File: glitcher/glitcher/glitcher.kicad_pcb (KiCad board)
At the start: 4 copper layers, 165.1 x 96.5 mm, 81 parts, among them J1 Barrel_Jack, J2 Conn_01x06, J3 Conn_01x03, J4 Conn_01x03, J5 Conn_01x03, J6 Conn_01x03, J7 Conn_01x03, SW1_1V8_OUT1 SW_DPDT_x2, SW2_1V2_OUT1 SW_DPDT_x2, SW3_VADJ_OUT1 SW_DPDT_x2, SW4_3V3_OUT1 SW_DPDT_x2, SW5_2V5_OUT1 SW_DPDT_x2, U1 SC0915, U2 CMOD_A7, U3 max4619cpe+, U4_1V8_OUT1 LD1117S18TR_SOT223, U5_1V2_OUT1 LD1117S12TR_SOT223, U6_VADJ_OUT1 NCP1117-ADJ_SOT223, U7_3V3_OUT1 LD1117S33TR_SOT223, U8_2V5_OUT1 LD1117S25TR_SOT223, U9_3V3ALWAYS1 LD1117S33TR_SOT223

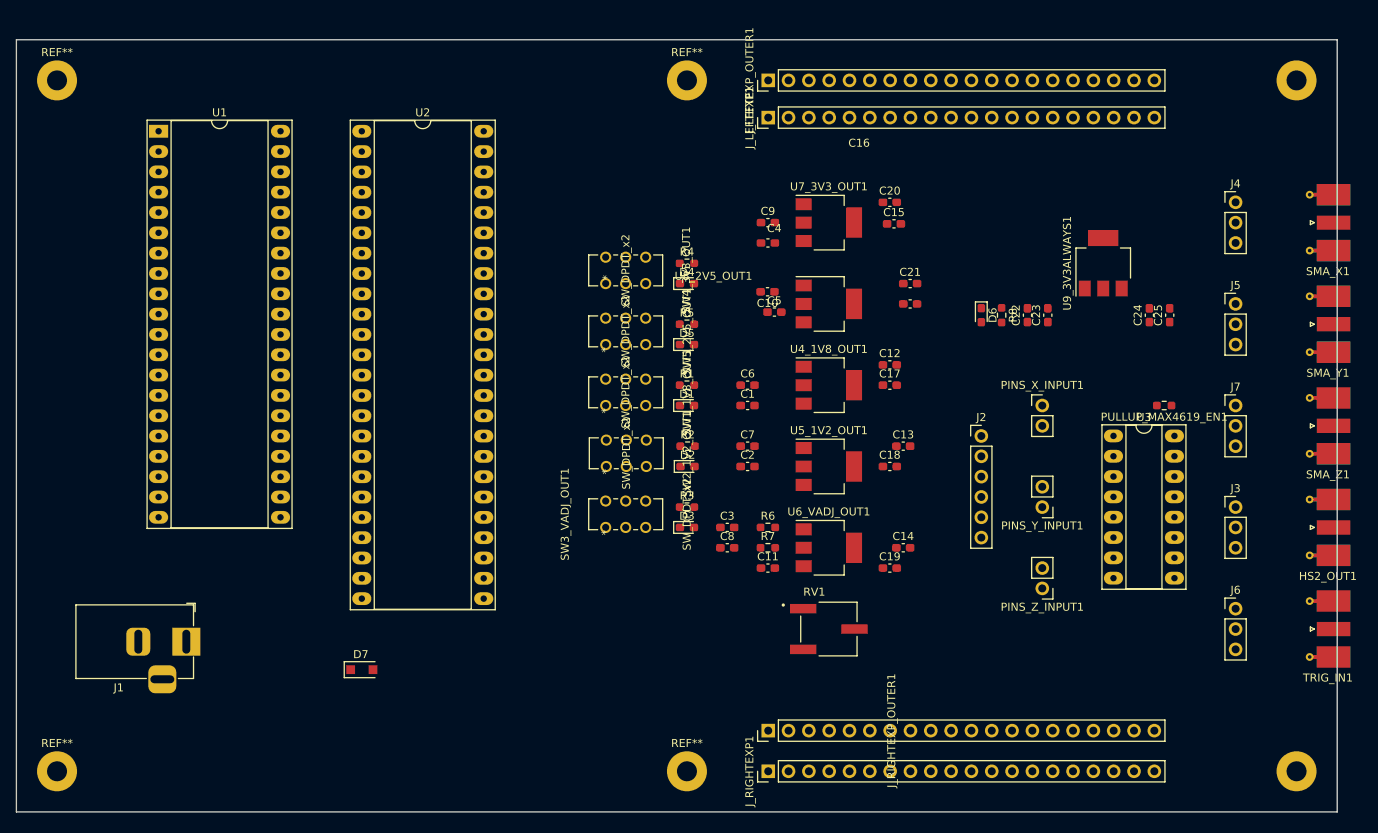
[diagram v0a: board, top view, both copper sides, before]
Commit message: lolsave
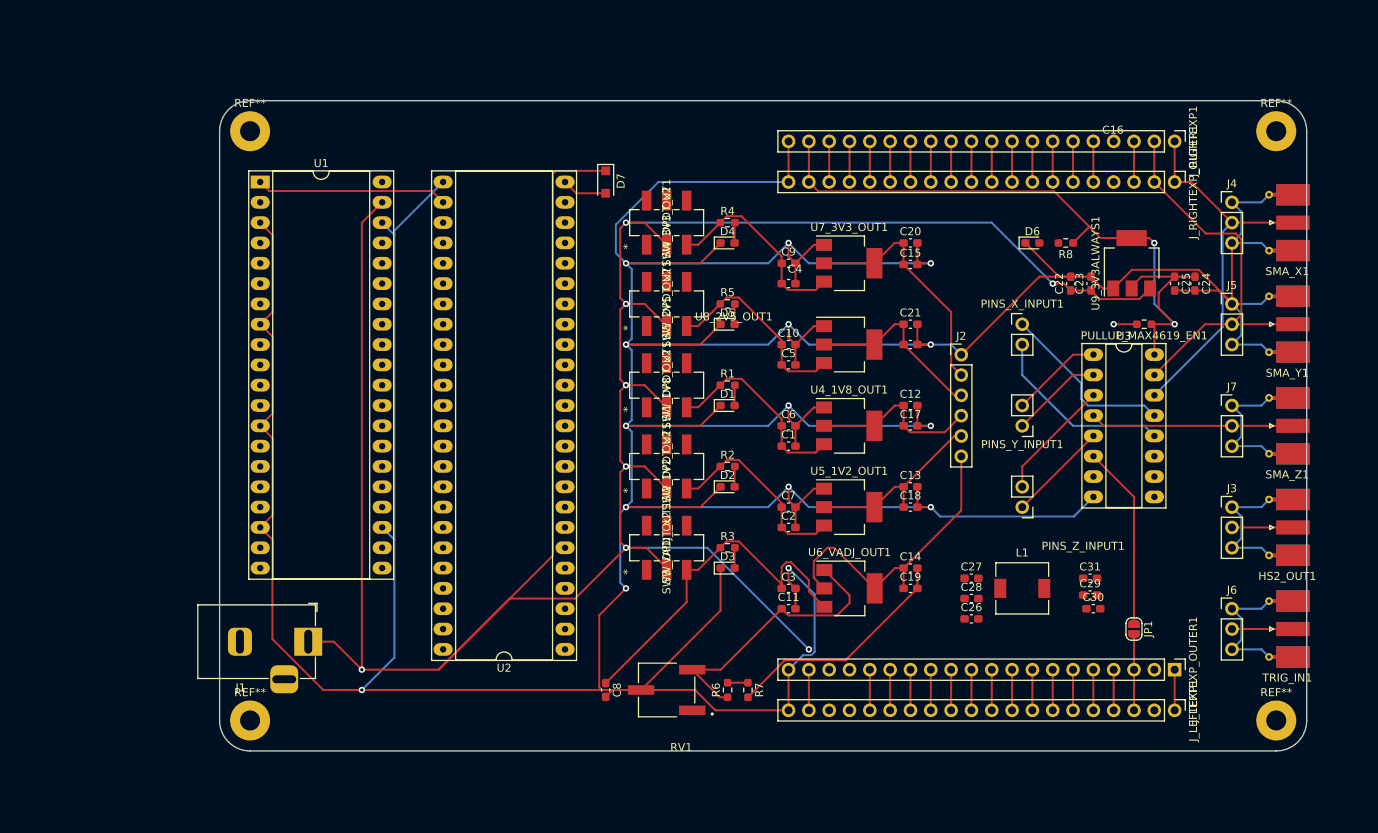
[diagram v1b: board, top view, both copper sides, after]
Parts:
- removed ? (x2): , 
- removed the REF** at (170.2, 38.1)
- removed the REF** at (91.4, 38.1)
- removed the REF** at (170.2, 124.5)
- removed the REF** at (91.4, 124.5)
- added C26: C, Capacitor_SMD:C_0603_1608Metric_Pad1.08x0.95mm_HandSolder, F.Cu at (205.7, 105.4)
- added C27: C, Capacitor_SMD:C_0603_1608Metric_Pad1.08x0.95mm_HandSolder, F.Cu at (205.7, 100.3)
- added C28: C, Capacitor_SMD:C_0603_1608Metric_Pad1.08x0.95mm_HandSolder, F.Cu at (205.7, 102.9)
- added C29: C, Capacitor_SMD:C_0603_1608Metric_Pad1.08x0.95mm_HandSolder, F.Cu at (220.6, 102.4)
- added C30: C, Capacitor_SMD:C_0603_1608Metric_Pad1.08x0.95mm_HandSolder, F.Cu at (221.0, 104.1)
- added C31: C, Capacitor_SMD:C_0603_1608Metric_Pad1.08x0.95mm_HandSolder, F.Cu at (220.6, 100.3)
- added JP1: SolderJumper_2_Open, Jumper:SolderJumper-2_P1.3mm_Open_RoundedPad1.0x1.5mm, F.Cu at (226.1, 106.7)
- added L1: INDUCTOR, Inductor_SMD:L_6.3x6.3_H3, F.Cu at (212.1, 101.6)
- added REF**: MountingHole_2.5mm_Pad, MountingHole:MountingHole_2.5mm_Pad, F.Cu at (243.8, 118.1)
- added REF**: MountingHole_2.5mm_Pad, MountingHole:MountingHole_2.5mm_Pad, F.Cu at (243.8, 44.5)
- added REF**: MountingHole_2.5mm_Pad, MountingHole:MountingHole_2.5mm_Pad, F.Cu at (115.6, 44.5)
- added REF**: MountingHole_2.5mm_Pad, MountingHole:MountingHole_2.5mm_Pad, F.Cu at (115.6, 118.1)
- SW1_1V8_OUT1, SW2_1V2_OUT1, SW3_VADJ_OUT1, SW4_3V3_OUT1, SW5_2V5_OUT1: footprint all_lib:SW_JS202011CQN -> all_lib:JS202011SCQN
- moved J_RIGHTEXP1 93.7 mm to (231.1, 45.7), turned to -90 degrees
- moved J_LEFTEXP1 89.8 mm to (231.1, 116.8), turned to -90 degrees
- moved J_LEFTEXP_OUTER1 89.5 mm to (231.1, 111.8), turned to -90 degrees
- moved J_RIGHTEXP_OUTER1 85.3 mm to (231.1, 50.8), turned to -90 degrees
- moved U2 69.6 mm to (154.9, 109.2), turned to 180 degrees
- moved D7 68.1 mm to (160.0, 50.8), turned to -90 degrees
- moved C8 23.4 mm to (160.0, 114.3), turned to -90 degrees
- moved RV1 21.7 mm to (167.6, 114.3), turned to 180 degrees
- moved R6 20.9 mm to (175.3, 114.3), turned to 90 degrees
- moved R7 18.0 mm to (177.8, 114.3), turned to -90 degrees
- moved J1 15.2 mm to (122.8, 108.3)
- moved U1 14.2 mm to (116.8, 50.8)
- moved R8 12.1 mm to (217.5, 58.4), turned to 180 degrees
- moved D6 11.1 mm to (213.4, 58.4), turned to 0 degrees
- moved C3 10.8 mm to (182.9, 101.6)
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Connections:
- D7 pad 1: unconnected-(D7-Pad1) -> VCC
- D7 pad 2: unconnected-(D7-Pad2) -> Net-(D7-Pad2)
- J_LEFTEXP1 pad 1: unconnected-(J_LEFTEXP1-Pad1) -> GND
- J_LEFTEXP1 pad 10: unconnected-(J_LEFTEXP1-Pad10) -> RPI_GP9
- J_LEFTEXP1 pad 11: unconnected-(J_LEFTEXP1-Pad11) -> RPI_GP10
- J_LEFTEXP1 pad 12: unconnected-(J_LEFTEXP1-Pad12) -> RPI_GP11
- J_LEFTEXP1 pad 13: unconnected-(J_LEFTEXP1-Pad13) -> RPI_GP12
- J_LEFTEXP1 pad 14: unconnected-(J_LEFTEXP1-Pad14) -> RPI_GP13
- J_LEFTEXP1 pad 15: unconnected-(J_LEFTEXP1-Pad15) -> RPI_GP14
- J_LEFTEXP1 pad 16: unconnected-(J_LEFTEXP1-Pad16) -> RPI_GP15
- J_LEFTEXP1 pad 19: unconnected-(J_LEFTEXP1-Pad19) -> VCC
- J_LEFTEXP1 pad 20: unconnected-(J_LEFTEXP1-Pad20) -> GND
- J_LEFTEXP1 pad 3: unconnected-(J_LEFTEXP1-Pad3) -> RPI_GP2
- J_LEFTEXP1 pad 4: unconnected-(J_LEFTEXP1-Pad4) -> RPI_GP3
- J_LEFTEXP1 pad 5: unconnected-(J_LEFTEXP1-Pad5) -> RPI_GP4
- J_LEFTEXP1 pad 6: unconnected-(J_LEFTEXP1-Pad6) -> RPI_GP5
- J_LEFTEXP1 pad 7: unconnected-(J_LEFTEXP1-Pad7) -> RPI_GP6
- J_LEFTEXP1 pad 8: unconnected-(J_LEFTEXP1-Pad8) -> RPI_GP7
- J_LEFTEXP1 pad 9: unconnected-(J_LEFTEXP1-Pad9) -> RPI_GP8
- J_LEFTEXP_OUTER1 pad 1: unconnected-(J_LEFTEXP_OUTER1-Pad1) -> GND
- J_LEFTEXP_OUTER1 pad 10: unconnected-(J_LEFTEXP_OUTER1-Pad10) -> RPI_GP9
- J_LEFTEXP_OUTER1 pad 11: unconnected-(J_LEFTEXP_OUTER1-Pad11) -> RPI_GP10
- J_LEFTEXP_OUTER1 pad 12: unconnected-(J_LEFTEXP_OUTER1-Pad12) -> RPI_GP11
- J_LEFTEXP_OUTER1 pad 13: unconnected-(J_LEFTEXP_OUTER1-Pad13) -> RPI_GP12
- J_LEFTEXP_OUTER1 pad 14: unconnected-(J_LEFTEXP_OUTER1-Pad14) -> RPI_GP13
- J_LEFTEXP_OUTER1 pad 15: unconnected-(J_LEFTEXP_OUTER1-Pad15) -> RPI_GP14
- J_LEFTEXP_OUTER1 pad 16: unconnected-(J_LEFTEXP_OUTER1-Pad16) -> RPI_GP15
- J_LEFTEXP_OUTER1 pad 19: unconnected-(J_LEFTEXP_OUTER1-Pad19) -> VCC
- J_LEFTEXP_OUTER1 pad 20: unconnected-(J_LEFTEXP_OUTER1-Pad20) -> GND
- J_LEFTEXP_OUTER1 pad 3: unconnected-(J_LEFTEXP_OUTER1-Pad3) -> RPI_GP2
- J_LEFTEXP_OUTER1 pad 4: unconnected-(J_LEFTEXP_OUTER1-Pad4) -> RPI_GP3
- J_LEFTEXP_OUTER1 pad 5: unconnected-(J_LEFTEXP_OUTER1-Pad5) -> RPI_GP4
- J_LEFTEXP_OUTER1 pad 6: unconnected-(J_LEFTEXP_OUTER1-Pad6) -> RPI_GP5
- J_LEFTEXP_OUTER1 pad 7: unconnected-(J_LEFTEXP_OUTER1-Pad7) -> RPI_GP6
- J_LEFTEXP_OUTER1 pad 8: unconnected-(J_LEFTEXP_OUTER1-Pad8) -> RPI_GP7
- J_LEFTEXP_OUTER1 pad 9: unconnected-(J_LEFTEXP_OUTER1-Pad9) -> RPI_GP8
- J_RIGHTEXP1 pad 1: unconnected-(J_RIGHTEXP1-Pad1) -> X_OUT
- J_RIGHTEXP1 pad 10: unconnected-(J_RIGHTEXP1-Pad10) -> FPGA_GPIO_10
- J_RIGHTEXP1 pad 11: unconnected-(J_RIGHTEXP1-Pad11) -> FPGA_GPIO_9
- J_RIGHTEXP1 pad 12: unconnected-(J_RIGHTEXP1-Pad12) -> FPGA_GPIO_8
- J_RIGHTEXP1 pad 13: unconnected-(J_RIGHTEXP1-Pad13) -> FPGA_GPIO_7
- J_RIGHTEXP1 pad 14: unconnected-(J_RIGHTEXP1-Pad14) -> FPGA_GPIO_6
- J_RIGHTEXP1 pad 15: unconnected-(J_RIGHTEXP1-Pad15) -> FPGA_GPIO_5
- J_RIGHTEXP1 pad 16: unconnected-(J_RIGHTEXP1-Pad16) -> FPGA_GPIO_4
- J_RIGHTEXP1 pad 17: unconnected-(J_RIGHTEXP1-Pad17) -> FPGA_GPIO_3
- J_RIGHTEXP1 pad 18: unconnected-(J_RIGHTEXP1-Pad18) -> FPGA_GPIO_2
- J_RIGHTEXP1 pad 19: unconnected-(J_RIGHTEXP1-Pad19) -> VCC_3V3_ALWAYS
- J_RIGHTEXP1 pad 2: unconnected-(J_RIGHTEXP1-Pad2) -> Y_OUT
- J_RIGHTEXP1 pad 20: unconnected-(J_RIGHTEXP1-Pad20) -> GND
- J_RIGHTEXP1 pad 3: unconnected-(J_RIGHTEXP1-Pad3) -> Z_OUT
- J_RIGHTEXP1 pad 5: unconnected-(J_RIGHTEXP1-Pad5) -> MAX4619_A
- J_RIGHTEXP1 pad 6: unconnected-(J_RIGHTEXP1-Pad6) -> MAX4619_B
- J_RIGHTEXP1 pad 7: unconnected-(J_RIGHTEXP1-Pad7) -> MAX4619_C
- J_RIGHTEXP1 pad 8: unconnected-(J_RIGHTEXP1-Pad8) -> FPGA_GPIO_12
- J_RIGHTEXP1 pad 9: unconnected-(J_RIGHTEXP1-Pad9) -> FPGA_GPIO_11
- J_RIGHTEXP_OUTER1 pad 1: unconnected-(J_RIGHTEXP_OUTER1-Pad1) -> X_OUT
- J_RIGHTEXP_OUTER1 pad 10: unconnected-(J_RIGHTEXP_OUTER1-Pad10) -> FPGA_GPIO_10
- J_RIGHTEXP_OUTER1 pad 11: unconnected-(J_RIGHTEXP_OUTER1-Pad11) -> FPGA_GPIO_9
- J_RIGHTEXP_OUTER1 pad 12: unconnected-(J_RIGHTEXP_OUTER1-Pad12) -> FPGA_GPIO_8
- J_RIGHTEXP_OUTER1 pad 13: unconnected-(J_RIGHTEXP_OUTER1-Pad13) -> FPGA_GPIO_7
- J_RIGHTEXP_OUTER1 pad 14: unconnected-(J_RIGHTEXP_OUTER1-Pad14) -> FPGA_GPIO_6
- J_RIGHTEXP_OUTER1 pad 15: unconnected-(J_RIGHTEXP_OUTER1-Pad15) -> FPGA_GPIO_5
- J_RIGHTEXP_OUTER1 pad 16: unconnected-(J_RIGHTEXP_OUTER1-Pad16) -> FPGA_GPIO_4
- J_RIGHTEXP_OUTER1 pad 17: unconnected-(J_RIGHTEXP_OUTER1-Pad17) -> FPGA_GPIO_3
- J_RIGHTEXP_OUTER1 pad 18: unconnected-(J_RIGHTEXP_OUTER1-Pad18) -> FPGA_GPIO_2
- J_RIGHTEXP_OUTER1 pad 19: unconnected-(J_RIGHTEXP_OUTER1-Pad19) -> VCC_3V3_ALWAYS
- J_RIGHTEXP_OUTER1 pad 2: unconnected-(J_RIGHTEXP_OUTER1-Pad2) -> Y_OUT
- J_RIGHTEXP_OUTER1 pad 20: unconnected-(J_RIGHTEXP_OUTER1-Pad20) -> GND
- J_RIGHTEXP_OUTER1 pad 3: unconnected-(J_RIGHTEXP_OUTER1-Pad3) -> Z_OUT
- J_RIGHTEXP_OUTER1 pad 5: unconnected-(J_RIGHTEXP_OUTER1-Pad5) -> MAX4619_A
- J_RIGHTEXP_OUTER1 pad 6: unconnected-(J_RIGHTEXP_OUTER1-Pad6) -> MAX4619_B
- J_RIGHTEXP_OUTER1 pad 7: unconnected-(J_RIGHTEXP_OUTER1-Pad7) -> MAX4619_C
- J_RIGHTEXP_OUTER1 pad 8: unconnected-(J_RIGHTEXP_OUTER1-Pad8) -> FPGA_GPIO_12
- J_RIGHTEXP_OUTER1 pad 9: unconnected-(J_RIGHTEXP_OUTER1-Pad9) -> FPGA_GPIO_11
- R8 pad 1: VCC -> VCC_3V3_ALWAYS
- U1 pad 1: unconnected-(U1-Pad1) -> RPI_GP0
- U1 pad 10: unconnected-(U1-Pad10) -> RPI_GP7
- U1 pad 11: unconnected-(U1-Pad11) -> RPI_GP8
- U1 pad 12: unconnected-(U1-Pad12) -> RPI_GP9
- U1 pad 14: unconnected-(U1-Pad14) -> RPI_GP10
- U1 pad 15: unconnected-(U1-Pad15) -> RPI_GP11
- U1 pad 16: unconnected-(U1-Pad16) -> RPI_GP12
- U1 pad 17: unconnected-(U1-Pad17) -> RPI_GP13
- U1 pad 19: unconnected-(U1-Pad19) -> RPI_GP14
- U1 pad 2: unconnected-(U1-Pad2) -> RPI_GP1
- U1 pad 20: unconnected-(U1-Pad20) -> RPI_GP15
- U1 pad 21: unconnected-(U1-Pad21) -> RPI_GP16
- U1 pad 22: unconnected-(U1-Pad22) -> RPI_GP17
- U1 pad 4: unconnected-(U1-Pad4) -> RPI_GP2
- U1 pad 5: unconnected-(U1-Pad5) -> RPI_GP3
- U1 pad 6: unconnected-(U1-Pad6) -> RPI_GP4
- U1 pad 7: unconnected-(U1-Pad7) -> RPI_GP5
- U1 pad 9: unconnected-(U1-Pad9) -> RPI_GP6
- U2 pad 1: unconnected-(U2-Pad1) -> MAX4619_C
- U2 pad 10: unconnected-(U2-Pad10) -> FPGA_GPIO_6
- U2 pad 11: unconnected-(U2-Pad11) -> FPGA_GPIO_5
- U2 pad 12: unconnected-(U2-Pad12) -> FPGA_GPIO_4
- U2 pad 13: unconnected-(U2-Pad13) -> FPGA_GPIO_3
- U2 pad 14: unconnected-(U2-Pad14) -> FPGA_GPIO_2
- U2 pad 15: unconnected-(U2-Pad15) -> FPGA_GPIO_1
- U2 pad 2: unconnected-(U2-Pad2) -> MAX4619_B
- U2 pad 24: VCC -> Net-(D7-Pad2)
- U2 pad 26: unconnected-(U2-Pad26) -> RPI_GP0
- U2 pad 27: unconnected-(U2-Pad27) -> RPI_GP1
- U2 pad 3: unconnected-(U2-Pad3) -> MAX4619_A
- U2 pad 4: unconnected-(U2-Pad4) -> FPGA_GPIO_12
- U2 pad 5: unconnected-(U2-Pad5) -> FPGA_GPIO_11
- U2 pad 6: unconnected-(U2-Pad6) -> FPGA_GPIO_10
- U2 pad 7: unconnected-(U2-Pad7) -> FPGA_GPIO_9
- U2 pad 8: unconnected-(U2-Pad8) -> FPGA_GPIO_8
- U2 pad 9: unconnected-(U2-Pad9) -> FPGA_GPIO_7
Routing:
- net GND: track 0.00 -> 871.1 mm, vias 0 -> 15
- net VCC: track 0.00 -> 361.6 mm, vias 0 -> 8
- net RPI_GP2: track 0.00 -> 140.8 mm
- net RPI_GP3: track 0.00 -> 132.8 mm
- net MAX4619_C: track 0.00 -> 131.3 mm
- net RPI_GP4: track 0.00 -> 130.3 mm
- net RPI_GP5: track 0.00 -> 127.8 mm
- net MAX4619_B: track 0.00 -> 127.7 mm
- net MAX4619_A: track 0.00 -> 124.3 mm
- net RPI_GP6: track 0.00 -> 121.0 mm
- net RPI_GP7: track 0.00 -> 117.4 mm
- net RPI_GP8: track 0.00 -> 114.9 mm
- net RPI_GP9: track 0.00 -> 110.2 mm
- net RPI_GP10: track 0.00 -> 105.6 mm
- net RPI_GP11: track 0.00 -> 102.0 mm
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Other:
- board size 165.1 x 96.5 mm -> 135.9 x 81.3 mm
